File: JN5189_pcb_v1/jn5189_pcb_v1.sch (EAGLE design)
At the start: 25 parts, among them Y1 32.768KHz, Y2 32Mhz

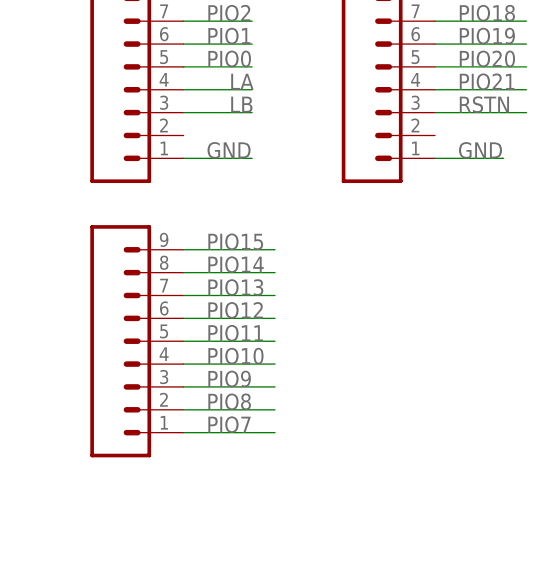
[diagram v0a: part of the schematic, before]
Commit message: Add files via upload
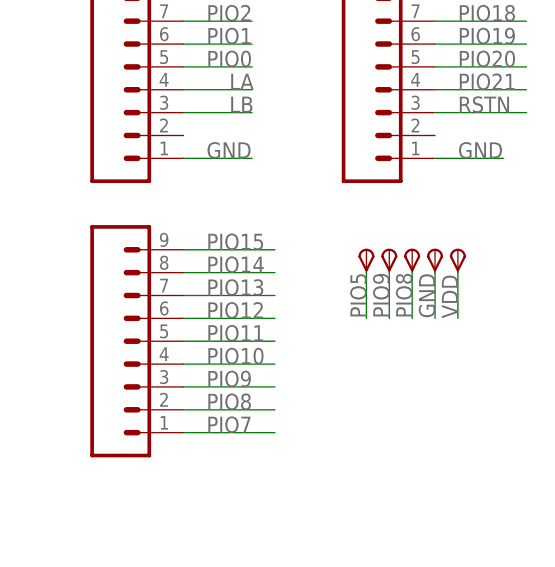
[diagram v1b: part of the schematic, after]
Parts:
- added 3V3, GND, ISP, RXD, TXD: TPSTP11R, testpad:TPSTP11R
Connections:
- net GND: now also GND.PP
- net PIO5: now also ISP.PP
- net PIO8: now also TXD.PP
- net PIO9: now also RXD.PP
- net VDD: now also 3V3.PP
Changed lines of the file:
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@@
 <part name="GND14" library="supply1" library_urn="urn:adsk.eagle:library:371" deviceset="GND" device=""/>
 <part name="GND15" library="supply1" library_urn="urn:adsk.eagle:library:371" deviceset="GND" device=""/>
+<part name="GND" library="testpad" library_urn="urn:adsk.eagle:library:385" deviceset="TPS" device="TP11R" package3d_urn="urn:adsk.eagle:package:27961/1" value="TPSTP11R"/>
+<part name="3V3" library="testpad" library_urn="urn:adsk.eagle:library:385" deviceset="TPS" device="TP11R" package3d_urn="urn:adsk.eagle:package:27961/1" value="TPSTP11R"/>
+<part name="RXD" library="testpad" library_urn="urn:adsk.eagle:library:385" deviceset="TPS" device="TP11R" package3d_urn="urn:adsk.eagle:package:27961/1" value="TPSTP11R"/>
+<part name="ISP" library="testpad" library_urn="urn:adsk.eagle:library:385" deviceset="TPS" device="TP11R" package3d_urn="urn:adsk.eagle:package:27961/1" value="TPSTP11R"/>
+<part name="TXD" library="testpad" library_urn="urn:adsk.eagle:library:385" deviceset="TPS" device="TP11R" package3d_urn="urn:adsk.eagle:package:27961/1" value="TPSTP11R"/>
 </parts>
 <sheets>
@@
 <instance part="GND15" gate="1" x="167.64" y="2.54" smashed="yes">
 <attribute name="VALUE" x="165.1" y="0" size="1.778" layer="96"/>
+</instance>
+<instance part="GND" gate="G$1" x="281.94" y="48.26" smashed="yes">
+<attribute name="TP_SIGNAL_NAME" x="283.21" y="46.99" size="1.778" layer="97"/>
+</instance>
+<instance part="3V3" gate="G$1" x="284.48" y="48.26" smashed="yes">
+<attribute name="TP_SIGNAL_NAME" x="285.75" y="46.99" size="1.778" layer="97"/>
+</instance>
+<instance part="RXD" gate="G$1" x="276.86" y="48.26" smashed="yes">
+<attribute name="TP_SIGNAL_NAME" x="278.13" y="46.99" size="1.778" layer="97"/>
+</instance>
+<instance part="ISP" gate="G$1" x="274.32" y="48.26" smashed="yes">
+<attribute name="TP_SIGNAL_NAME" x="275.59" y="46.99" size="1.778" layer="97"/>
+</instance>
+<instance part="TXD" gate="G$1" x="279.4" y="48.26" smashed="yes">
+<attribute name="TP_SIGNAL_NAME" x="280.67" y="46.99" size="1.778" layer="97"/>
 </instance>
 </instances>
@@
 <wire x1="254" y1="58.42" x2="261.62" y2="58.42" width="0.1524" layer="91"/>
 <label x="256.54" y="58.42" size="1.778" layer="95"/>
+</segment>
+<segment>
+<pinref part="GND" gate="G$1" pin="PP"/>
+<wire x1="281.94" y1="45.72" x2="281.94" y2="40.64" width="0.1524" layer="91"/>
+<label x="281.94" y="40.64" size="1.778" layer="95" rot="R90"/>
 </segment>
 </net>
@@
 <label x="284.48" y="81.28" size="1.778" layer="95"/>
 </segment>
+<segment>
+<pinref part="3V3" gate="G$1" pin="PP"/>
+<wire x1="284.48" y1="45.72" x2="284.48" y2="40.64" width="0.1524" layer="91"/>
+<label x="284.48" y="40.64" size="1.778" layer="95" rot="R90"/>
+</segment>
 </net>
 <net name="N$1" class="0">
@@
 <label x="256.54" y="33.02" size="1.778" layer="95"/>
 </segment>
+<segment>
+<pinref part="RXD" gate="G$1" pin="PP"/>
+<wire x1="276.86" y1="45.72" x2="276.86" y2="40.64" width="0.1524" layer="91"/>
+<label x="276.86" y="40.64" size="1.778" layer="95" rot="R90"/>
+</segment>
 </net>
 <net name="PIO8" class="0">
@@
 <label x="256.54" y="30.48" size="1.778" layer="95"/>
 </segment>
+<segment>
+<pinref part="TXD" gate="G$1" pin="PP"/>
+<wire x1="279.4" y1="45.72" x2="279.4" y2="40.64" width="0.1524" layer="91"/>
+<label x="279.4" y="40.64" size="1.778" layer="95" rot="R90"/>
+</segment>
 </net>
 <net name="PIO7" class="0">
@@
 <label x="256.54" y="81.28" size="1.778" layer="95"/>
 </segment>
-</net>
+<segment>
+<pinref part="ISP" gate="G$1" pin="PP"/>
+<wire x1="274.32" y1="45.72" x2="274.32" y2="40.64" width="0.1524" layer="91"/>
+<label x="274.32" y="40.64" size="1.778" layer="95" rot="R90"/>
+</segment>
+</net>
